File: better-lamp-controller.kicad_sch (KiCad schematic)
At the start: 23 parts, among them J1 Conn_02x20_Odd_Even, J4 Conn_02x10_Odd_Even, J5 Conn_01x05_Pin, J6 Conn_01x02_Pin, J7 Conn_01x04_Pin, J8 Conn_01x04_Pin, U1 LP5860T, U2 DRV8837C, U4 MAX98360A, U6 74AHCT1G08

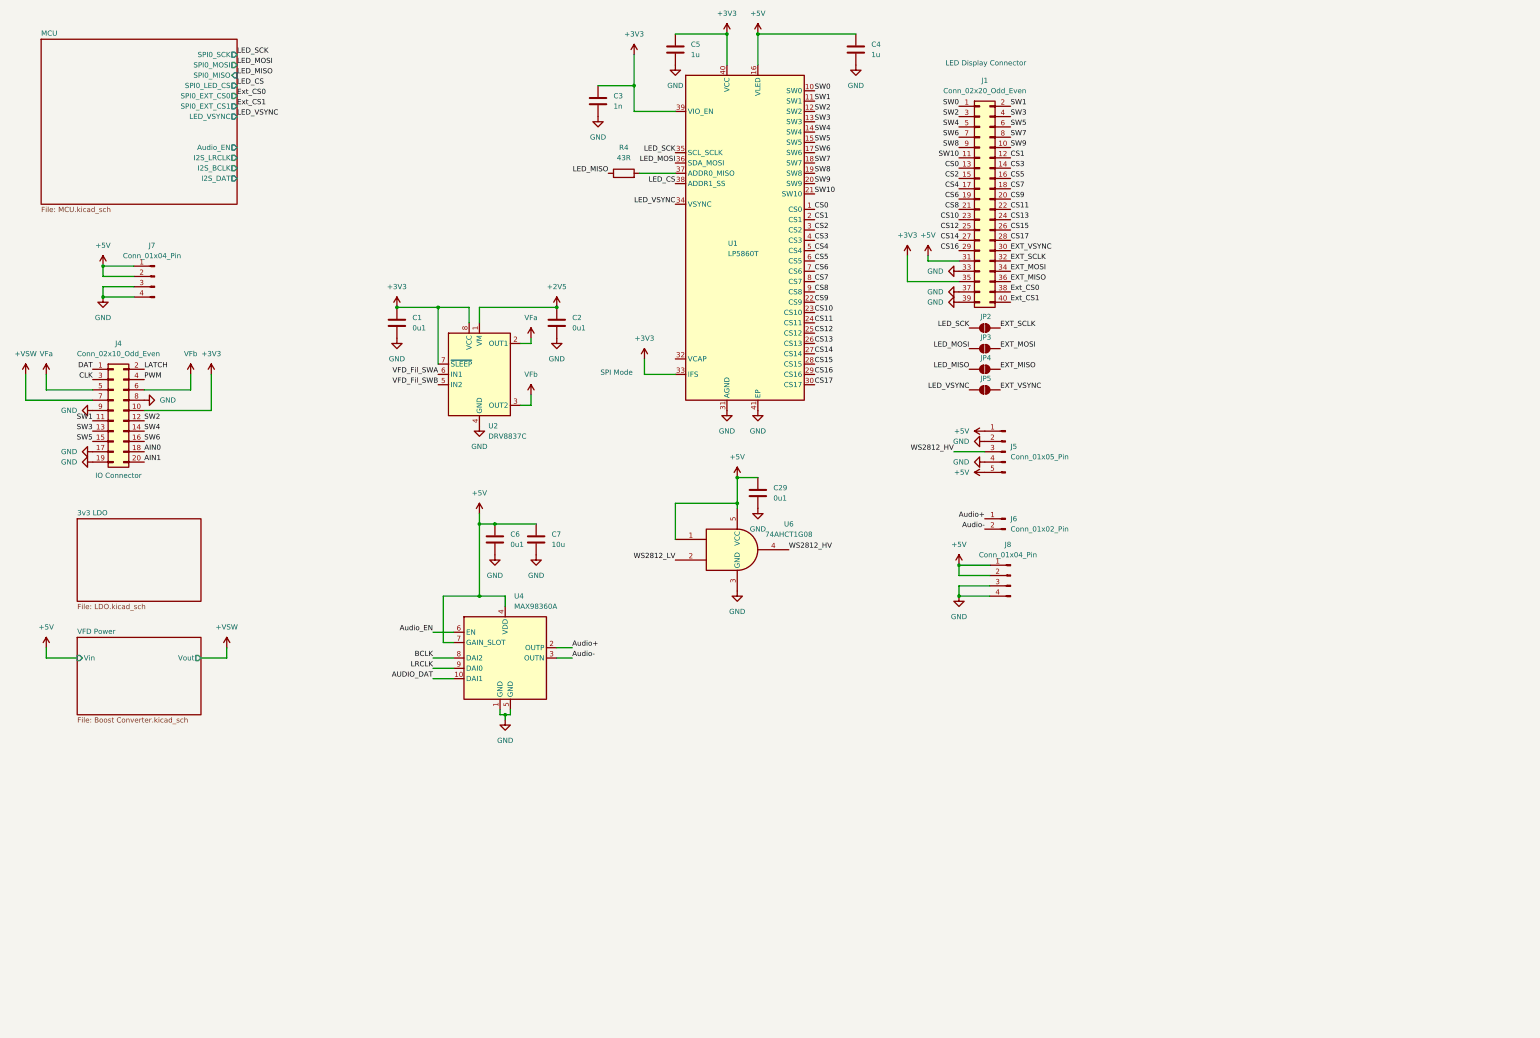
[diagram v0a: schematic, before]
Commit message: Add RTC
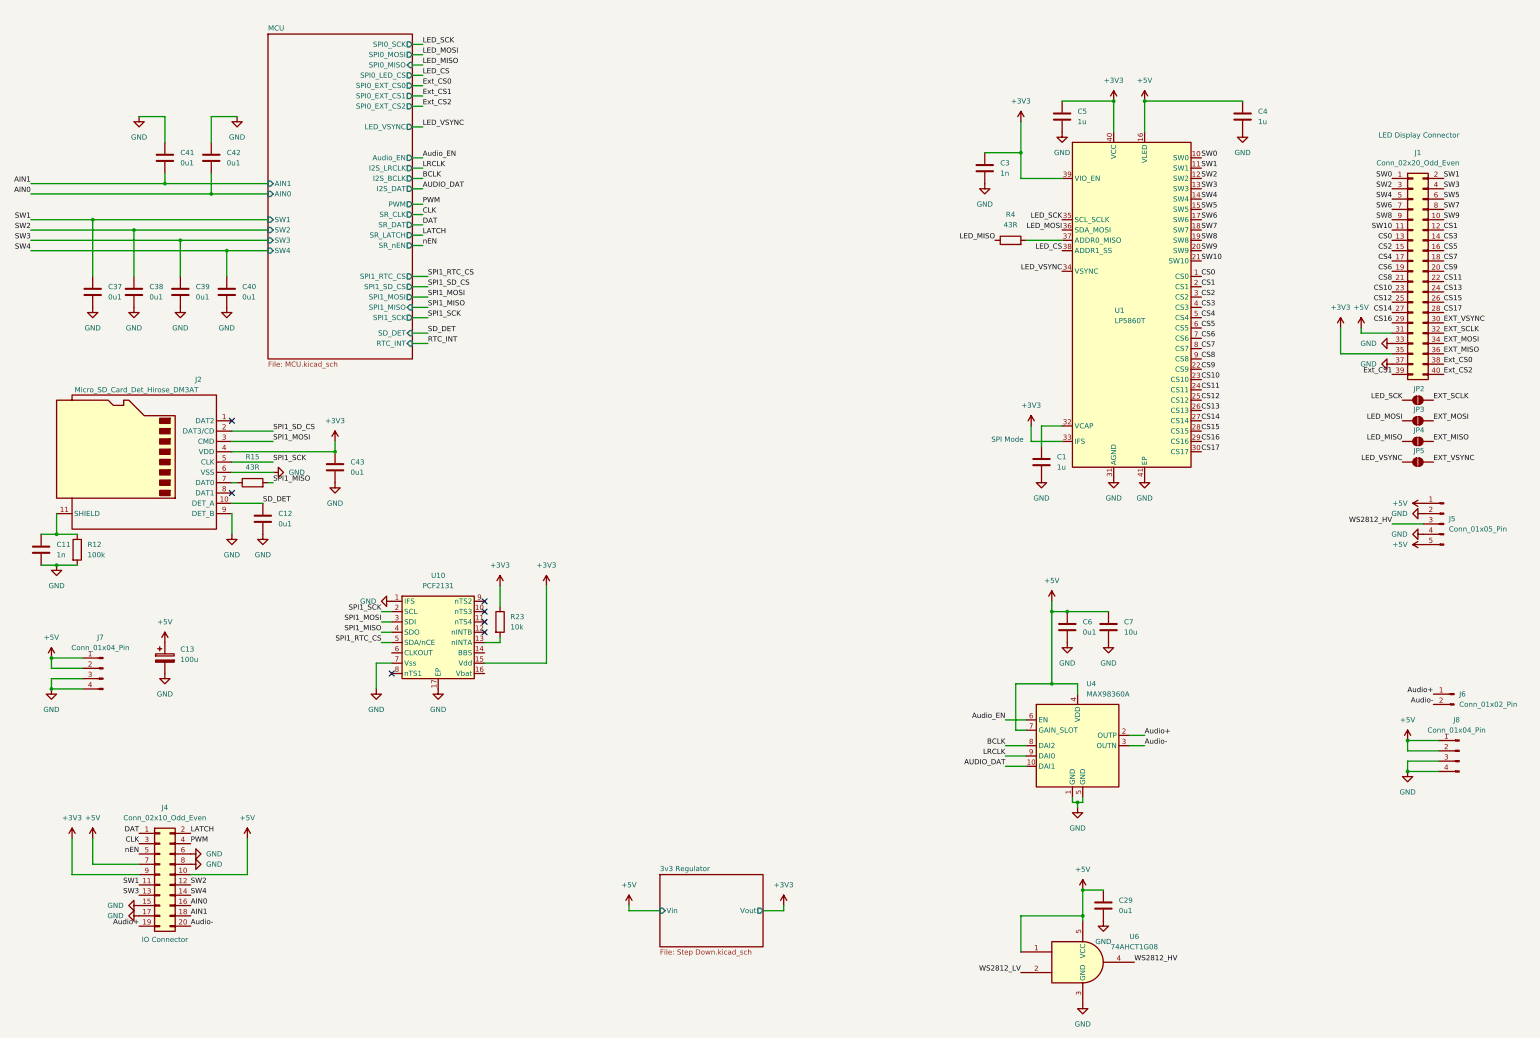
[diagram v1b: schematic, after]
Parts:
- removed C2: 0u1, symbol Device:C
- removed U2: DRV8837C, Package_SON:WSON-8-1EP_2x2mm_P0.5mm_EP0.9x1.6mm, symbol Driver_Motor:DRV8837C
- added C11: 1n, Capacitor_SMD:C_0603_1608Metric_Pad1.08x0.95mm_HandSolder, symbol Device:C
- added C12, C37, C38, C39, C40, C41, C42, C43: 0u1, Capacitor_SMD:C_0603_1608Metric_Pad1.08x0.95mm_HandSolder, symbol Device:C
- added C13: 100u, Capacitor_THT:CP_Radial_D10.0mm_P5.00mm, symbol Device:C_Polarized
- added J2: Micro_SD_Card_Det_Hirose_DM3AT, Connector_Card:microSD_HC_Hirose_DM3AT-SF-PEJM5, symbol Connector:Micro_SD_Card_Det_Hirose_DM3AT
- added R12: 100k, Resistor_SMD:R_0603_1608Metric_Pad0.98x0.95mm_HandSolder, symbol Device:R
- added R15: 43R, Resistor_SMD:R_0603_1608Metric_Pad0.98x0.95mm_HandSolder, symbol Device:R
- added R23: 10k, Resistor_SMD:R_0603_1608Metric_Pad0.98x0.95mm_HandSolder, symbol Device:R
- added U10: PCF2131, kicad global library:HLSON16_SOT1992-1, symbol Global:PCF2131
- C1: value 0u1 -> 1u; footprint (none) -> Capacitor_SMD:C_0805_2012Metric_Pad1.18x1.45mm_HandSolder
- C29, C3, C6: footprint (none) -> Capacitor_SMD:C_0603_1608Metric_Pad1.08x0.95mm_HandSolder
- C4, C5: footprint (none) -> Capacitor_SMD:C_0805_2012Metric_Pad1.18x1.45mm_HandSolder
- C7: footprint (none) -> Capacitor_SMD:C_1210_3225Metric
- J1: footprint (none) -> Connector_IDC:IDC-Header_2x20_P2.54mm_Vertical
- J4: footprint (none) -> Connector_IDC:IDC-Header_2x10_P2.54mm_Vertical
- J5: footprint (none) -> Connector_PinHeader_2.54mm:PinHeader_1x05_P2.54mm_Vertical
- J6: footprint (none) -> Connector_PinHeader_2.54mm:PinHeader_1x02_P2.54mm_Vertical
- J7, J8: footprint (none) -> Connector_PinHeader_2.54mm:PinHeader_1x04_P2.54mm_Vertical
- JP2, JP3, JP4, JP5: footprint (none) -> Jumper:SolderJumper-2_P1.3mm_Open_RoundedPad1.0x1.5mm
- R4: footprint (none) -> Resistor_SMD:R_0603_1608Metric_Pad0.98x0.95mm_HandSolder
- U6: footprint (none) -> Package_TO_SOT_SMD:SOT-23-5
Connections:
- net +VSW is gone; now on net +5V: J4.7 (Pin_7)
- net VFb is gone; now on net GND: J4.6 (Pin_6)
- net +3V3: now also J4.9 (Pin_9), C43.1, J2.4 (VDD), R23.1, U10.15 (Vdd); no longer C1.1, J4.10 (Pin_10)
- net +5V: now also J4.10 (Pin_10), C13.1
- net AIN0: now also J4.16 (Pin_16), C42.2; no longer J4.18 (Pin_18)
- net AIN1: now also J4.18 (Pin_18), C41.2; no longer J4.20 (Pin_20)
- net Audio+: now also J4.19 (Pin_19)
- net Audio-: now also J4.20 (Pin_20)
- net Ext_CS1: now also J1.39 (Pin_39); no longer J1.40 (Pin_40)
- net GND: now also J4.15 (Pin_15), C11.2, C12.2, C13.2, C37.2, C38.2, C39.2, C40.2, C41.1, C42.1, C43.2, J2.6 (VSS), J2.9 (DET_B), R12.2, U10.1 (IFS), U10.17 (EP), U10.7 (Vss); no longer J1.39 (Pin_39), J4.19 (Pin_19), J4.9 (Pin_9)
- net SW1: now also C37.1
- net SW2: now also C38.1
- net SW3: now also C39.1
- net SW4: now also C40.1
- net SW5: no longer J4.15 (Pin_15)
- net SW6: no longer J4.16 (Pin_16)
- net at U1.32 (VCAP): now also C1.1
- net VFa renamed nEN
- new net: C11.1, J2.11 (SHIELD), R12.1
- new net: J2.7 (DAT0), R15.1
- new net: R23.2, U10.13 (nINTA)
- new net Ext_CS2: J1.40 (Pin_40)
- new net SD_DET: C12.1, J2.10 (DET_A)
- new net SPI1_MISO: R15.2, U10.4 (SDO)
- new net SPI1_MOSI: J2.3 (CMD), U10.3 (SDI)
- new net SPI1_RTC_CS: U10.5 (SDA/nCE)
- new net SPI1_SCK: J2.5 (CLK), U10.2 (SCL)
- new net SPI1_SD_CS: J2.2 (DAT3/CD)
- no-connect marks 0 -> 7
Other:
- removed sheet 3v3 LDO
- removed sheet VFD Power
- added sheet 3v3 Regulator (Step Down.kicad_sch)
- sheet MCU ports: added AIN0, AIN1, PWM, RTC_INT, SD_DET, SPI0_EXT_CS2, SPI1_MISO, SPI1_MOSI, SPI1_RTC_CS, SPI1_SCK, SPI1_SD_CS, SR_CLK, SR_DAT, SR_LATCH, SR_nEN, SW1, SW2, SW3, SW4; removed none
- moved on the sheet: C29, C3, C4, C5, C6, C7, J1, J4, J5, J6, J7, J8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
